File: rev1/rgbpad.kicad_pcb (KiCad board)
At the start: 2 copper layers, 100 x 100 mm, 102 parts, among them P1 CONN_01X06_TOP, P2 CONN_01X06_LEFT, P3 CONN_01X06_RIGHT, P4 CONN_01X06_BOTTOM, P5 CONN_01X07_DEBUG, SW1 SW_PUSH_2X2, SW2 SW_PUSH_2X2, SW3 SW_PUSH_2X2, SW4 SW_PUSH_2X2, SW5 SW_PUSH_RST, U1 STM32F030C8Tx, U10 APA102, U11 APA102, U12 APA102, U13 APA102, U14 APA102, U15 APA102, U16 APA102, U17 APA102, U2 APA102, U3 APA102, U4 APA102, U5 APA102, U6 APA102, U7 APA102, U8 APA102, U9 APA102

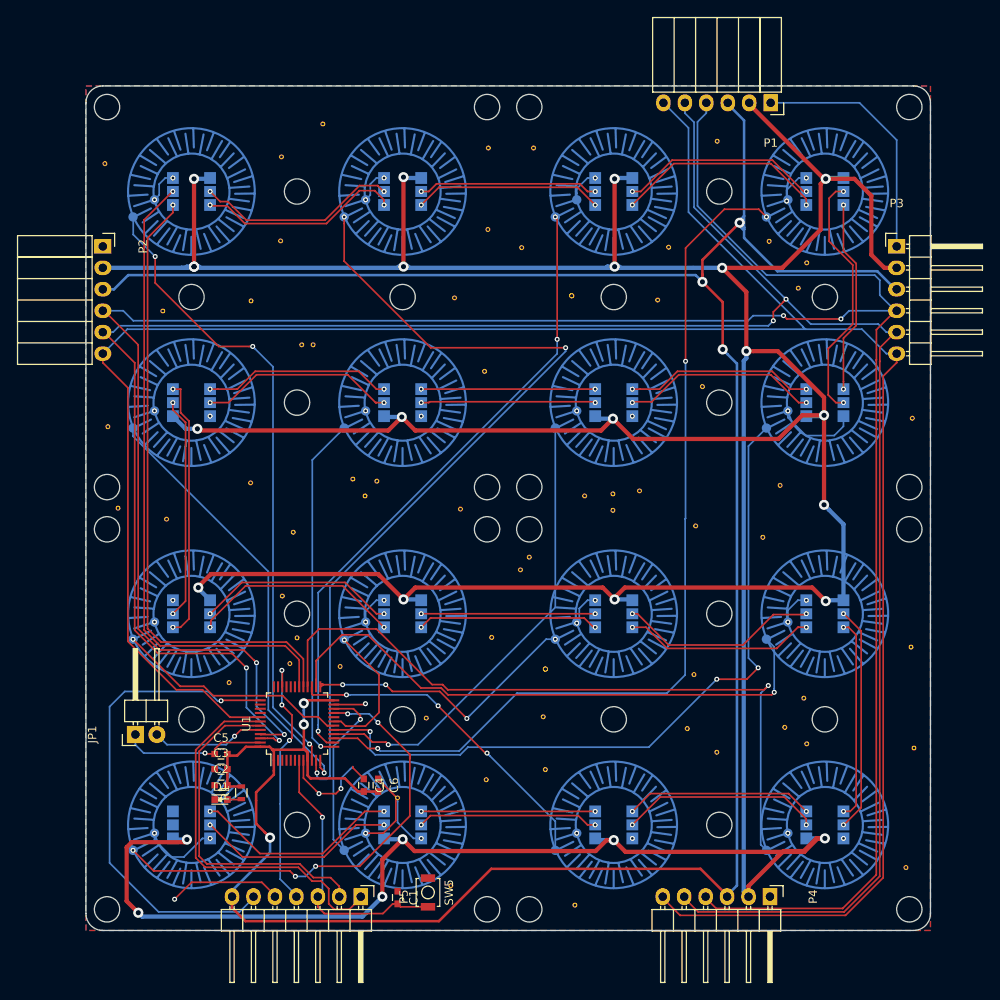
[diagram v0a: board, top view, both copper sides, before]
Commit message: New PCB layout
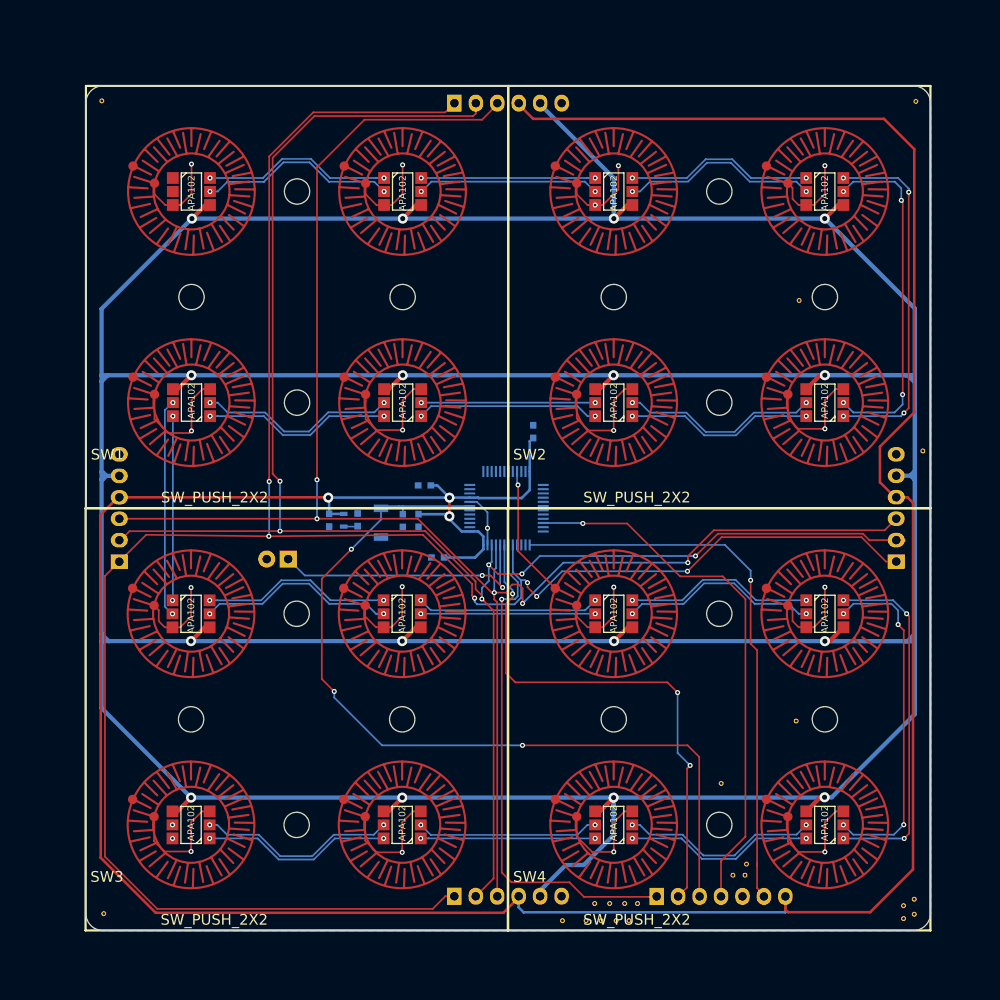
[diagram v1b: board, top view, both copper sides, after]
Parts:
- removed the REF** at (117.7, 75.3)
- removed the REF** at (130.9, 68.4)
- removed the REF** at (80.1, 118.8)
- removed the REF** at (74.2, 118.4)
- removed the REF** at (74.5, 102.8)
- removed the REF** at (59.5, 101.3)
- removed the REF** at (104.2, 124.7)
- removed the REF** at (103.0, 57.4)
- removed the REF** at (97.7, 57.4)
- removed the REF** at (132.2, 97.3)
- removed the REF** at (130.2, 103.5)
- removed the REF** at (119.0, 69.1)
- removed the REF** at (124.7, 128.9)
- removed the REF** at (135.0, 122.5)
- removed the REF** at (135.3, 127.9)
- removed the REF** at (147.1, 142.6)
- removed the REF** at (107.9, 147.0)
- removed the REF** at (104.4, 130.9)
- removed the REF** at (97.4, 132.2)
- removed the REF** at (69.5, 97.0)
- removed the REF** at (52.2, 59.2)
- removed the REF** at (59.1, 76.7)
- removed the REF** at (90.3, 124.8)
- removed the REF** at (134.3, 74.0)
- removed the REF** at (52.6, 90.3)
- removed the REF** at (104.4, 119.0) (x2)
- removed the REF** at (124.8, 56.5)
- removed the REF** at (148.1, 128.4)
- removed the REF** at (147.7, 116.5)
- removed the REF** at (147.8, 89.3)
- removed the REF** at (132.8, 126.0)
- removed the REF** at (122.0, 119.7)
- removed the REF** at (93.2, 144.7)
- removed the REF** at (121.2, 126.1)
- removed the REF** at (122.2, 102.1)
- removed the REF** at (78.0, 54.5)
- removed the REF** at (73.2, 58.4)
- removed the REF** at (73.0, 68.3)
- removed the REF** at (97.6, 67.0)
- removed the REF** at (101.6, 69.2)
- removed the REF** at (107.5, 74.8) (x2)
- removed the REF** at (97.2, 83.8)
- removed the REF** at (75.0, 115.3)
- removed the REF** at (93.7, 75.1)
- removed the REF** at (69.5, 75.5)
- removed the REF** at (101.5, 107.3)
- removed the REF** at (102.5, 105.8)
- removed the REF** at (112.4, 98.3)
- removed the REF** at (112.4, 100.2)
- removed the REF** at (115.5, 98.0)
- removed the REF** at (109.0, 98.5)
- removed the REF** at (83.0, 98.5)
- removed the REF** at (84.5, 96.8)
- removed the REF** at (73.2, 110.4)
- removed the REF** at (81.6, 96.5)
- removed the REF** at (76.9, 80.7)
- removed the REF** at (75.5, 80.7)
- removed the REF** at (98.0, 115.3)
- removed the REF** at (123.0, 85.6)
- removed the REF** at (94.3, 100.1)
- removed the REF** at (53.8, 100.0)
- removed the REF** at (67.0, 120.7)
- removed the REF** at (86.9, 134.3)
- removed the REF** at (135.3, 71.0)
- added REF**: VIA_0.6mm, assets:GND_VIA_0.6mm, F.Cu at (125.2, 132.6)
- added REF**: VIA_0.6mm, assets:GND_VIA_0.6mm, F.Cu at (114.3, 148.8)
- added REF**: VIA_0.6mm, assets:GND_VIA_0.6mm, F.Cu at (112.8, 148.8)
- added REF**: VIA_0.6mm, assets:GND_VIA_0.6mm, F.Cu at (111.0, 148.8)
- added REF**: VIA_0.6mm, assets:GND_VIA_0.6mm, F.Cu at (109.2, 148.8)
- added REF**: VIA_0.6mm, assets:GND_VIA_0.6mm, F.Cu at (106.4, 148.8)
- added REF**: VIA_0.6mm, assets:GND_VIA_0.6mm, F.Cu at (128.2, 142.1)
- added REF**: VIA_0.6mm, assets:GND_VIA_0.6mm, F.Cu at (128.0, 143.5)
- added REF**: VIA_0.6mm, assets:GND_VIA_0.6mm, F.Cu at (126.6, 143.5)
- added REF**: VIA_0.6mm, assets:GND_VIA_0.6mm, F.Cu at (148.3, 51.8)
- added REF**: VIA_0.6mm, assets:GND_VIA_0.6mm, F.Cu at (51.9, 51.8)
- added REF**: VIA_0.6mm, assets:GND_VIA_0.6mm, F.Cu at (146.8, 148.6)
- added REF**: VIA_0.6mm, assets:GND_VIA_0.6mm, F.Cu at (52.1, 148.0)
- added REF**: VIA_0.6mm, assets:GND_VIA_0.6mm, F.Cu at (134.4, 75.4)
- added REF**: VIA_0.6mm, assets:GND_VIA_0.6mm, F.Cu at (134.1, 125.2)
- added REF**: VIA_0.6mm, assets:GND_VIA_0.6mm, F.Cu at (148.1, 148.1)
- added REF**: VIA_0.6mm, assets:GND_VIA_0.6mm, F.Cu at (148.1, 146.3)
- added REF**: VIA_0.6mm, assets:GND_VIA_0.6mm, F.Cu at (146.8, 147.1)
- added REF**: VIA_0.6mm, assets:GND_VIA_0.6mm, F.Cu at (149.1, 93.2)
- added REF**: VIA_0.6mm, assets:GND_VIA_0.6mm, F.Cu at (110.2, 146.8)
- added REF**: VIA_0.6mm, assets:GND_VIA_0.6mm, F.Cu at (115.3, 146.8)
- added REF**: VIA_0.6mm, assets:GND_VIA_0.6mm, F.Cu at (113.8, 146.8)
- added REF**: VIA_0.6mm, assets:GND_VIA_0.6mm, F.Cu at (112.0, 146.8)
- C1, C2, C3, C4, C5, C6, D1, JP1, P1, P2, P3, P4, P5, R1, SW5, U1: moved to B.Cu
- SW1, SW2, SW3, SW4, U10, U11, U12, U13, U14, U15, U16, U17, U2, U3, U4, U5, U6, U7, U8, U9: moved to F.Cu
- moved C3 54.4 mm to (103.0, 90.9), turned to 270 degrees
- moved C1 44.6 mm to (87.5, 101.5), turned to 90 degrees
- moved SW5 44.1 mm to (84.9, 101.7), turned to 90 degrees
- moved C2 42.9 mm to (90.1, 97.3)
- moved P1 37.5 mm to (93.6, 52.0), turned to 0 degrees
- moved P2 37.4 mm to (54.0, 106.3), turned to 90 degrees
- moved P4 37.4 mm to (93.6, 145.9)
- moved P3 37.3 mm to (145.9, 106.3)
- moved D1 36.9 mm to (82.2, 101.4), turned to 270 degrees
- moved U1 35.6 mm to (99.8, 100.0), turned to 0 degrees
- moved SW1 35.4 mm to (75.0, 75.0)
- moved SW2 35.4 mm to (125.0, 75.0)
- moved SW4 35.4 mm to (125.0, 125.0)
- moved SW3 35.3 mm to (75.0, 125.0)
- moved P5 35.0 mm to (117.6, 146.0)
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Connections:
- JP1 pad 1: GND -> /STM32 controller/BOOT0
- JP1 pad 2: /STM32 controller/BOOT0 -> GND
- P1 pad 1: GND -> /STM32 controller/NINT
- P1 pad 2: +5V -> /STM32 controller/I2C_SDA
- P1 pad 3: +3V3 -> /STM32 controller/I2C_SCL
- P1 pad 4: /STM32 controller/I2C_SCL -> +3V3
- P1 pad 5: /STM32 controller/I2C_SDA -> +5V
- P1 pad 6: /STM32 controller/NINT -> GND
- P2 pad 1: GND -> /STM32 controller/NINT
- P2 pad 2: +5V -> /STM32 controller/I2C_SDA
- P2 pad 3: +3V3 -> /STM32 controller/I2C_SCL
- P2 pad 4: /STM32 controller/I2C_SCL -> +3V3
- P2 pad 5: /STM32 controller/I2C_SDA -> +5V
- P2 pad 6: /STM32 controller/NINT -> GND
- P3 pad 1: GND -> /STM32 controller/NINT
- P3 pad 2: +5V -> /STM32 controller/I2C_SDA
- P3 pad 3: +3V3 -> /STM32 controller/I2C_SCL
- P3 pad 4: /STM32 controller/I2C_SCL -> +3V3
- P3 pad 5: /STM32 controller/I2C_SDA -> +5V
- P3 pad 6: /STM32 controller/NINT -> GND
- P4 pad 1: GND -> /STM32 controller/NINT
- P4 pad 2: +5V -> /STM32 controller/I2C_SDA
- P4 pad 3: +3V3 -> /STM32 controller/I2C_SCL
- P4 pad 4: /STM32 controller/I2C_SCL -> +3V3
- P4 pad 5: /STM32 controller/I2C_SDA -> +5V
- P4 pad 6: /STM32 controller/NINT -> GND
- SW1 pad 5: /STM32 controller/BTN3 -> /STM32 controller/BTN5
- SW1 pad 7: /STM32 controller/BTN4 -> /STM32 controller/BTN6
- SW2 pad 1: /STM32 controller/BTN5 -> /STM32 controller/BTN3
- SW2 pad 3: /STM32 controller/BTN6 -> /STM32 controller/BTN4
- SW3 pad 5: /STM32 controller/BTN11 -> /STM32 controller/BTN13
- SW3 pad 7: /STM32 controller/BTN12 -> /STM32 controller/BTN14
- SW4 pad 1: /STM32 controller/BTN13 -> /STM32 controller/BTN11
- SW4 pad 3: /STM32 controller/BTN14 -> /STM32 controller/BTN12
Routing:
- net /STM32 controller/BTN6: track 108.4 -> 0.00 mm, vias 3 -> 0
- net /STM32 controller/BTN2: track 101.8 -> 0.00 mm, vias 3 -> 0
- net /STM32 controller/BTN8: track 86.7 -> 0.00 mm, vias 3 -> 0
- net /STM32 controller/I2C_SCL: track 296.0 -> 211.0 mm, vias 4 -> 5
- net /STM32 controller/BTN16: track 84.0 -> 0.00 mm, vias 1 -> 0
- net /4x4_LED/CIN: track 76.4 -> 0.00 mm, vias 1 -> 0
- net /STM32 controller/BTN1: track 75.5 -> 0.00 mm, vias 3 -> 0
- net /STM32 controller/BTN5: track 75.3 -> 0.00 mm, vias 3 -> 0
- net /4x4_LED/DIN: track 74.6 -> 0.00 mm, vias 1 -> 0
- net /STM32 controller/BTN14: track 68.3 -> 0.00 mm, vias 1 -> 0
- net /STM32 controller/I2C_SDA: track 282.1 -> 214.2 mm, vias 4 -> 6
- net /STM32 controller/NRST: track 32.7 -> 100.5 mm, vias 1 -> 3
- net GND: track 141.1 -> 201.6 mm, vias 35 -> 18
- net /STM32 controller/BTN7: track 54.7 -> 0.00 mm, vias 1 -> 0
- net /STM32 controller/BTN3: track 51.9 -> 0.00 mm, vias 1 -> 0
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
